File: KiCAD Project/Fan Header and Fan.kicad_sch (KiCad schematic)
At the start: 7 parts, among them J2 B2B-XH-A(LF)(SN), J3 ESW-120-33-G-D, M1 CFM-2507CF-050-089, U7 CAT24C32HU4I-GT3

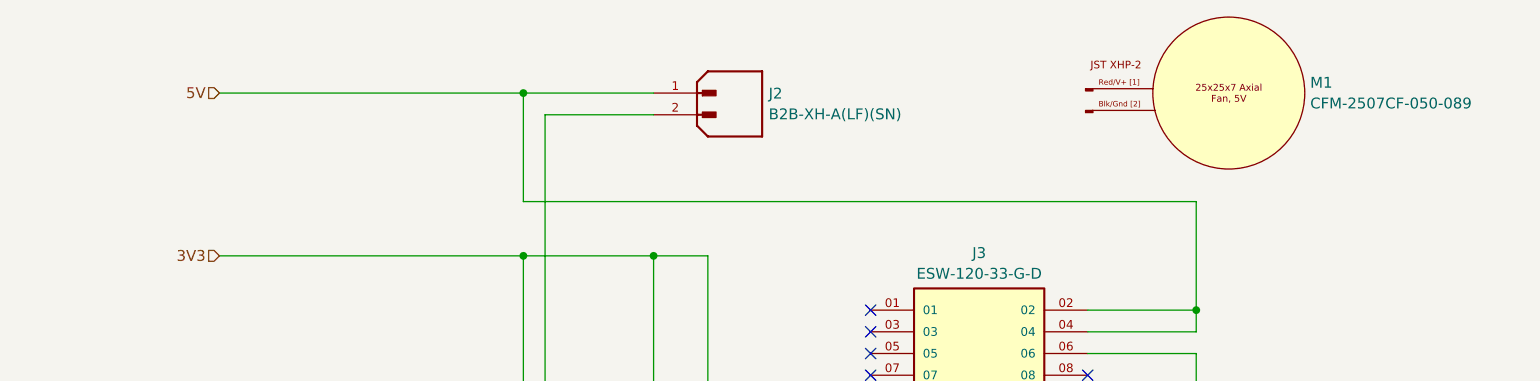
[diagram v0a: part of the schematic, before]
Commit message: v1.0.0 RC2
Build candidate 2
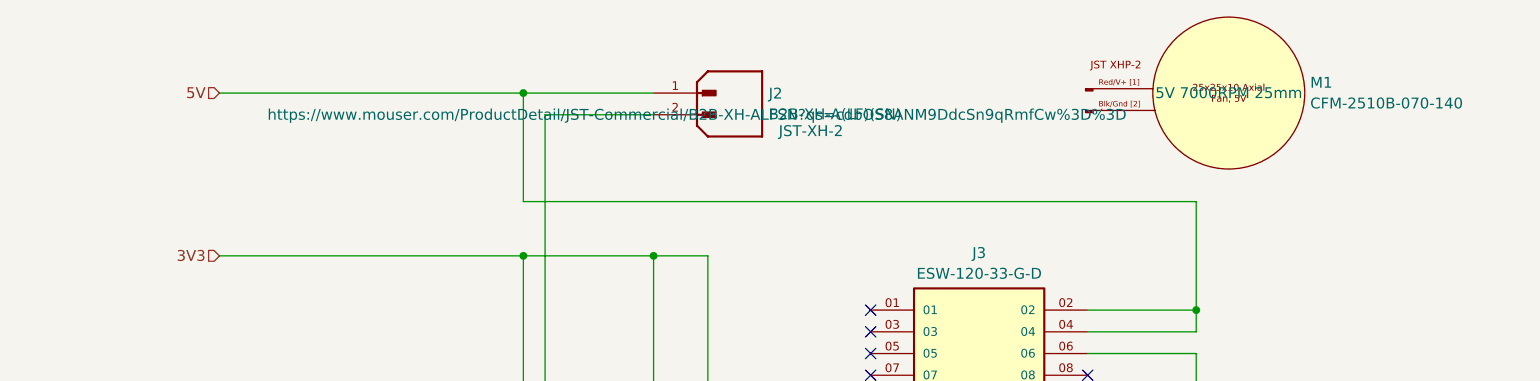
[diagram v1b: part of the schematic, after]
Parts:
- J2: Mouser Part Number (none) -> 306-B2BXHALFSNP; Mouser Price/Stock (none) -> https://www.mouser.com/ProductDetail/JST-Commercial/B2B-XH-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; Spec (none) -> JST-XH-2
- M1: value CFM-2507CF-050-089 -> CFM-2510B-070-140; footprint DW_Mechanical:[Fan] SameSky CFM-2507CF-050-089 -> DW_Mechanical:[Fan] SameSky CFM-2510B-070-140; symbol DW_Mechanical:[Fan] SameSky CFM-2507CF-050-089 -> DW_Mechanical:[Fan] SameSky CFM-2510B-070-140; Height 7 -> 10; Manufacturer_Part_Number CFM-2507CF-050-089 -> CFM-2510B-070-140; Mouser Part Number 179-CFM2507CF050089 -> 490-CFM2510B-070-140; Mouser Price/Stock https://www.mouser.com/ProductDetail/Same-Sky/CFM-2507CF-05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 -> https://www.mouser.com/ProductDetail/Same-Sky/CFM-2510B-070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; Spec (none) -> 5V 7000RPM 25mm
- U7: Spec (none) -> CAT24C32HU4I-GT3
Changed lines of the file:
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@@
 			)
 		)
-		(property "Spec" ""
+		(property "Spec" "CAT24C32HU4I-GT3"
 			(at 96.52 101.6 0)
 			(effects
@@
 		(on_board yes)
 		(dnp no)
-		(fields_autoplaced yes)
 		(property "Reference" "J2"
 			(at 155.702 50.8578 0)
@@
 			)
 		)
-		(property "Mouser Part Number" ""
+		(property "Mouser Part Number" "306-B2BXHALFSNP"
 			(at 147.32 53.34 0)
 			(effects
@@
 				)
 				(hide yes)
+			)
+		)
+		(property "Spec" "JST-XH-2"
+			(at 160.655 55.245 0)
+			(effects
+				(font
+					(size 1.27 1.27)
+				)
+			)
+		)
+		(property "Mouser Price/Stock" "https://www.mouser.com/ProductDetail/JST-Commercial/B2B-XH-ALFSN?qs=cdbOS8ANM9DdcSn9qRmfCw%3D%3D"
+			(at 147.32 53.34 0)
+			(effects
+				(font
+					(size 1.27 1.27)
+				)
 			)
 		)
@@
 	)
 	(symbol
-		(lib_id "DW_Mechanical:[Fan] SameSky CFM-2507CF-050-089")
+		(lib_id "DW_Mechanical:[Fan] SameSky CFM-2510B-070-140")
 		(at 209.55 50.8 0)
 		(unit 1)
@@
 			)
 		)
-		(property "Value" "CFM-2507CF-050-089"
+		(property "Value" "CFM-2510B-070-140"
 			(at 219.0749 52.0121 0)
 			(effects
@@
 			)
 		)
-		(property "Footprint" "DW_Mechanical:[Fan] SameSky CFM-2507CF-050-089"
+		(property "Footprint" "DW_Mechanical:[Fan] SameSky CFM-2510B-070-140"
 			(at 209.55 80.01 0)
 			(effects
@@
 			)
 		)
-		(property "Datasheet" "https://www.sameskydevices.com/product/resource/cfm-25cf.pdf"
+		(property "Datasheet" "https://www.sameskydevices.com/product/resource/cfm-25b.pdf"
 			(at 209.55 62.23 0)
 			(effects
@@
 			)
 		)
-		(property "Description" "DC Fans dc axial fan, 25 mm square, 7 mm, 5 Vdc, omniCOOL, 5000 RPM, 1.10 CFM"
+		(property "Description" "DC Fans dc axial fan, 25 mm square, 10 mm, 5 Vdc, omniCOOL, 5000 RPM, 1.35 CFM"
 			(at 209.55 74.93 0)
 			(effects
@@
 			)
 		)
-		(property "Height" "7"
+		(property "Height" "10"
 			(at 209.55 64.77 0)
 			(effects
@@
 			)
 		)
-		(property "Manufacturer_Part_Number" "CFM-2507CF-050-089"
+		(property "Manufacturer_Part_Number" "CFM-2510B-070-140"
 			(at 209.55 77.47 0)
 			(effects
@@
 			)
 		)
-		(property "Mouser Part Number" "179-CFM2507CF050089"
+		(property "Mouser Part Number" "490-CFM2510B-070-140"
 			(at 209.55 72.39 0)
 			(effects
@@
 			)
 		)
-		(property "Mouser Price/Stock" "https://www.mouser.com/ProductDetail/Same-Sky/CFM-2507CF-050-089?qs=ulEaXIWI0c9ptEGd6uhKEA%3D%3D"
+		(property "Mouser Price/Stock" "https://www.mouser.com/ProductDetail/Same-Sky/CFM-2510B-070-140?qs=GedFDFLaBXHD1VXBjs5CMA%3D%3D"
 			(at 209.55 69.85 0)
 			(effects
@@
 			)
 		)
+		(property "Spec" "5V 7000RPM 25mm"
+			(at 209.55 50.8 0)
+			(effects
+				(font
+					(size 1.27 1.27)
+				)
+			)
+		)
